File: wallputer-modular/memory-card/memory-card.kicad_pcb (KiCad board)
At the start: 2 copper layers, 99.7 x 99.7 mm, 1 part

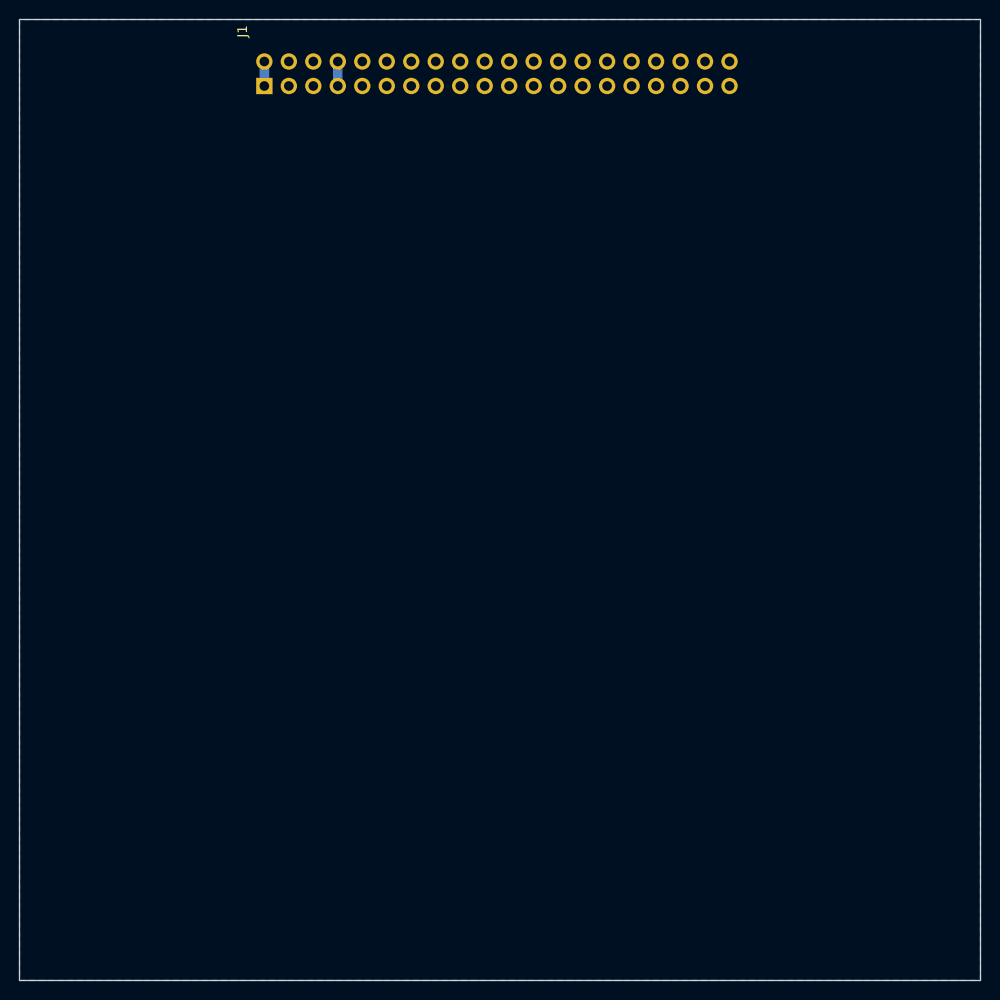
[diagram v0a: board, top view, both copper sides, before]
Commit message: begin wiring memory card
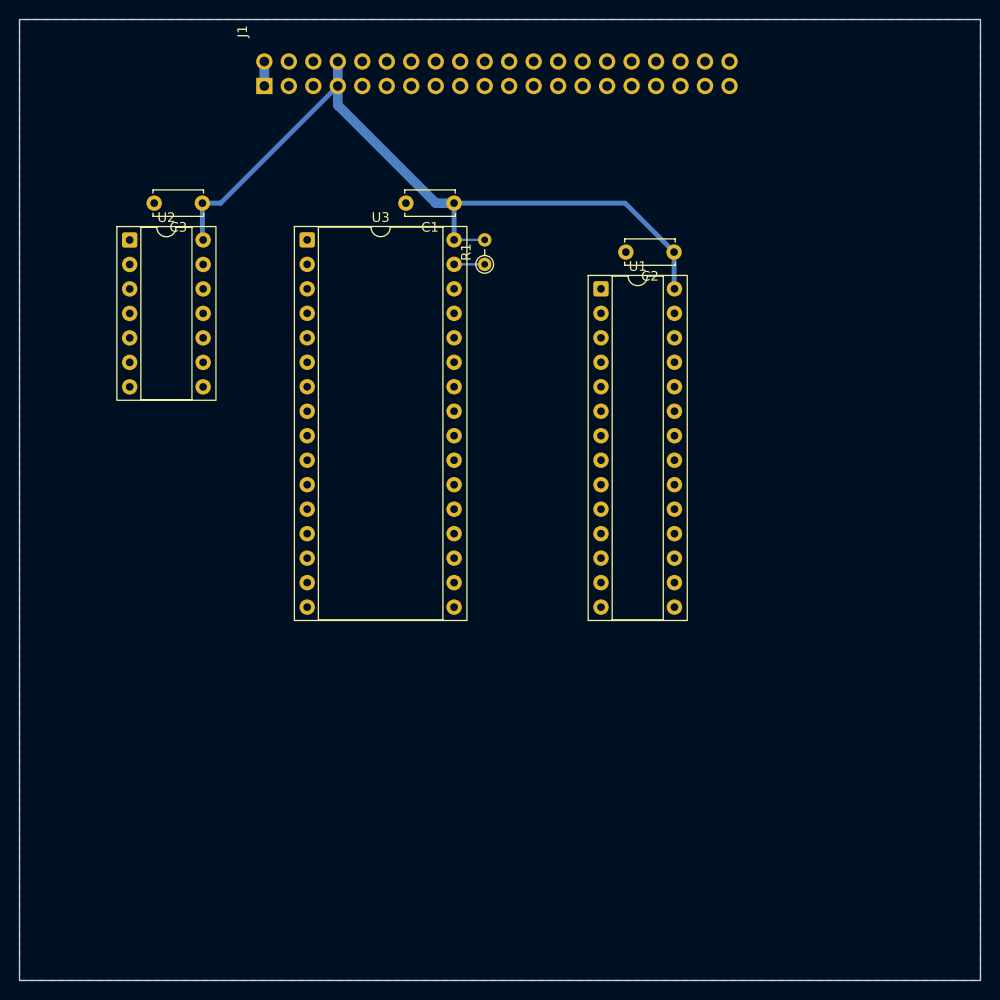
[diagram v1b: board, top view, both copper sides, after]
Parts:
- added C1: 100nF, Capacitor_THT:C_Disc_D5.0mm_W2.5mm_P5.00mm, F.Cu at (108.6, 82.5)
- added C2: 100nF, Capacitor_THT:C_Disc_D5.0mm_W2.5mm_P5.00mm, F.Cu at (131.4, 87.6)
- added C3: 100nF, Capacitor_THT:C_Disc_D5.0mm_W2.5mm_P5.00mm, F.Cu at (82.5, 82.5)
- added R1: 10k, Resistor_THT:R_Axial_DIN0204_L3.6mm_D1.6mm_P2.54mm_Vertical, F.Cu at (111.8, 88.9)
- added U1: HM62256BLP, Package_DIP:DIP-28_W7.62mm_Socket, F.Cu at (123.8, 91.4)
- added U2: 74HC00, Package_DIP:DIP-14_W7.62mm_Socket, F.Cu at (74.9, 86.4)
- added U3: SST39SF010, Package_DIP:DIP-32_W15.24mm_Socket, F.Cu at (93.3, 86.4)
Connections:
- J1 pad 10: unconnected-(J1-A5-Pad10) -> /A5
- J1 pad 11: unconnected-(J1-A6-Pad11) -> /A6
- J1 pad 12: unconnected-(J1-A7-Pad12) -> /A7
- J1 pad 13: unconnected-(J1-A8-Pad13) -> /A8
- J1 pad 14: unconnected-(J1-A9-Pad14) -> /A9
- J1 pad 15: unconnected-(J1-A10-Pad15) -> /A10
- J1 pad 16: unconnected-(J1-A11-Pad16) -> /A11
- J1 pad 17: unconnected-(J1-A12-Pad17) -> /A12
- J1 pad 18: unconnected-(J1-A13-Pad18) -> /A13
- J1 pad 19: unconnected-(J1-A14-Pad19) -> /A14
- J1 pad 20: unconnected-(J1-A15-Pad20) -> /A15
- J1 pad 21: unconnected-(J1-D0-Pad21) -> /D0
- J1 pad 22: unconnected-(J1-D1-Pad22) -> /D1
- J1 pad 23: unconnected-(J1-D2-Pad23) -> /D2
- J1 pad 24: unconnected-(J1-D3-Pad24) -> /D3
- J1 pad 25: unconnected-(J1-D4-Pad25) -> /D4
- J1 pad 26: unconnected-(J1-D5-Pad26) -> /D5
- J1 pad 27: unconnected-(J1-D6-Pad27) -> /D6
- J1 pad 28: unconnected-(J1-D7-Pad28) -> /D7
- J1 pad 29: unconnected-(J1-RW/-Pad29) -> RW/
- J1 pad 30: unconnected-(J1-NC-Pad30) -> ROM_PGM/
- J1 pad 35: unconnected-(J1-RAM/-Pad35) -> RAM/
- J1 pad 36: unconnected-(J1-ROM/-Pad36) -> ROM/
- J1 pad 38: unconnected-(J1-ACC/-Pad38) -> ACC/
- J1 pad 39: unconnected-(J1-CLK-Pad39) -> CLK
- J1 pad 5: unconnected-(J1-A0-Pad5) -> /A0
- J1 pad 6: unconnected-(J1-A1-Pad6) -> /A1
- J1 pad 7: unconnected-(J1-A2-Pad7) -> /A2
- J1 pad 8: unconnected-(J1-A3-Pad8) -> /A3
- J1 pad 9: unconnected-(J1-A4-Pad9) -> /A4
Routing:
- net +5V: track 2.54 -> 79.5 mm
- net ROM_PGM/: track 0.00 -> 3.18 mm
